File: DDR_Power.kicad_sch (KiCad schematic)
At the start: 10 parts, among them U6 NCP114AMX250TCG

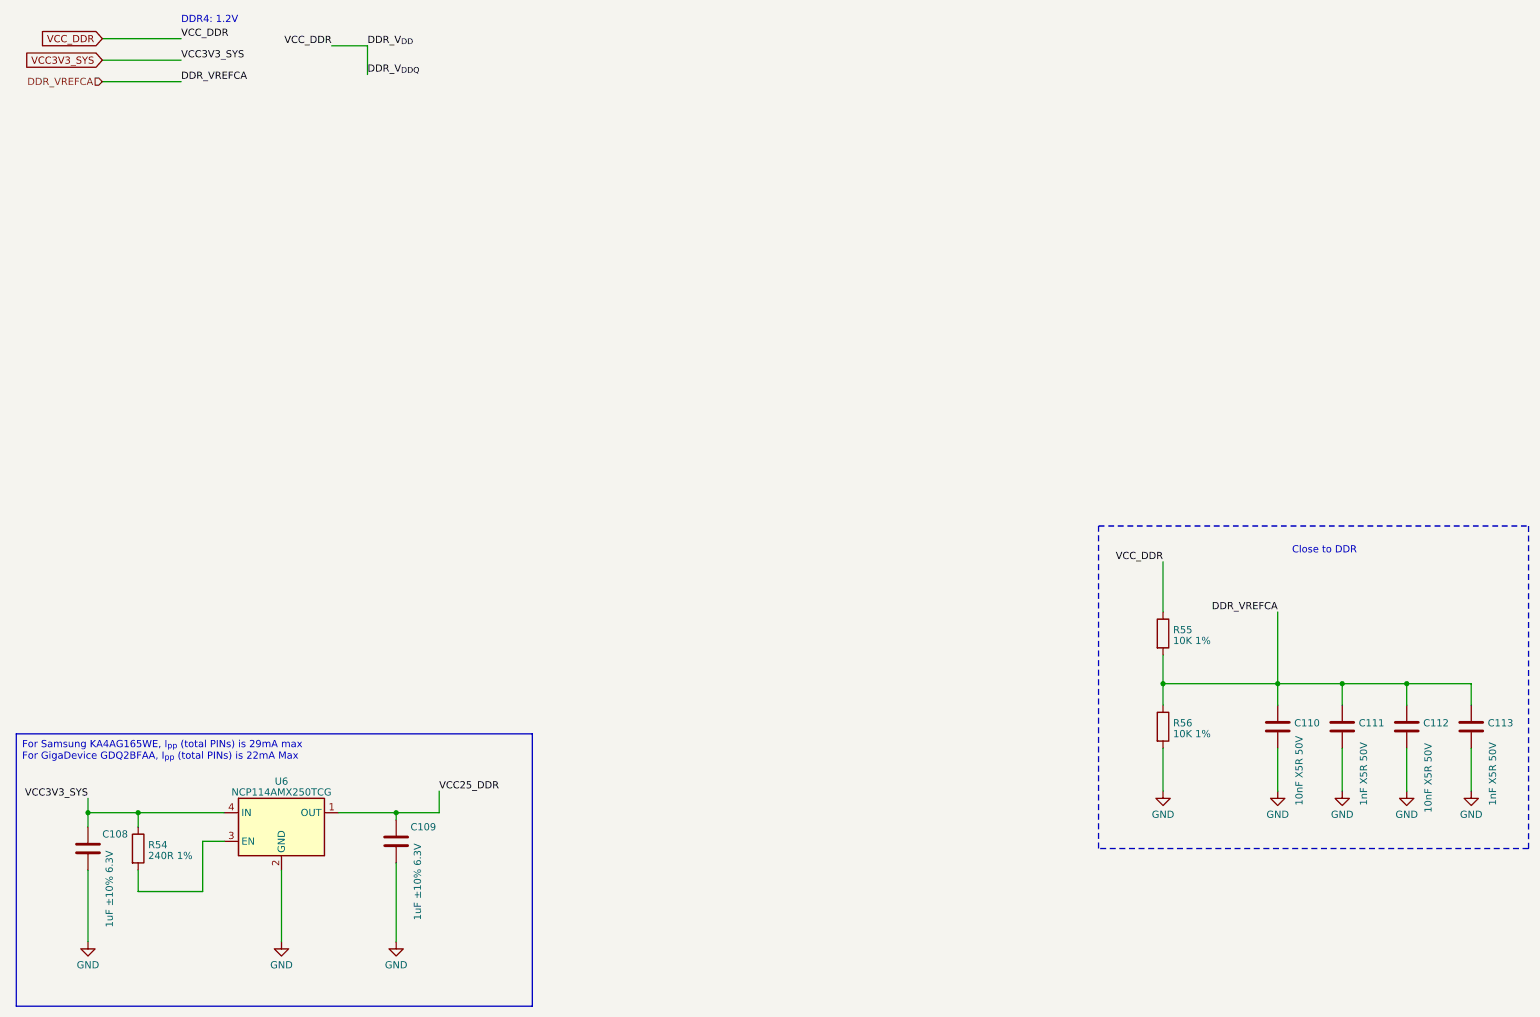
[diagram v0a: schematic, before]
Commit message: changed Power Label and copy DDR4 Sheets
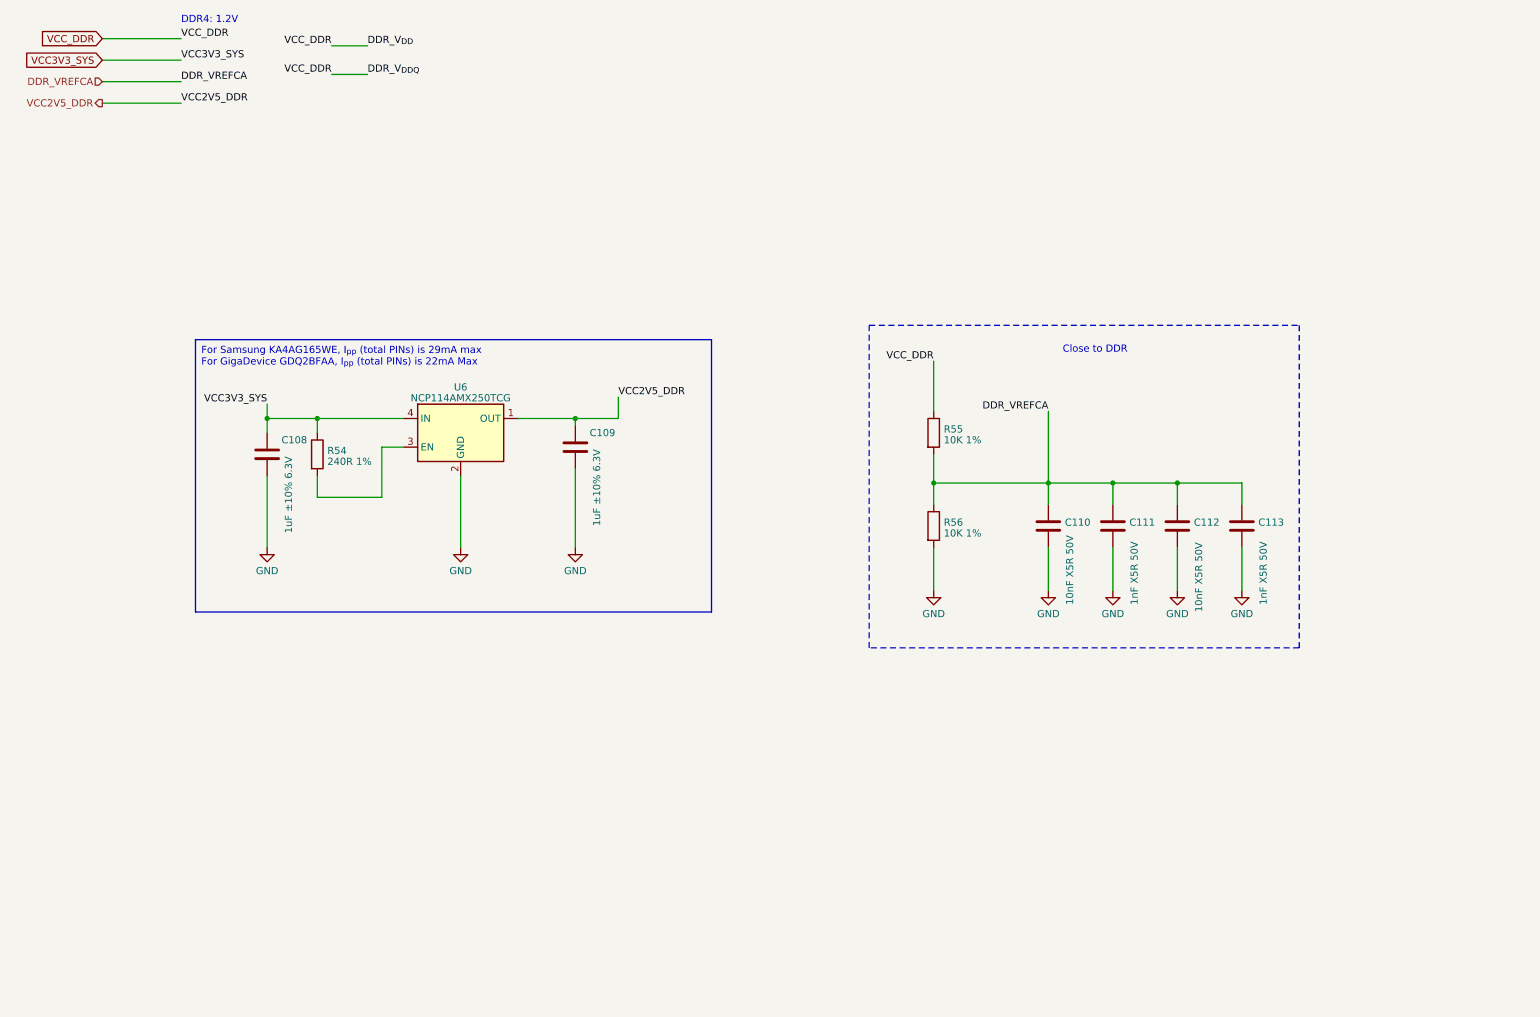
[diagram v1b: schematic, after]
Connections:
- net VCC25_DDR renamed VCC2V5_DDR
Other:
- moved on the sheet: C108, C109, C110, C111, C112, C113, R54, R55, R56, U6
